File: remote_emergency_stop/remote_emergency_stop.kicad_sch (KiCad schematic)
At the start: 20 parts, among them J1 Conn_01x02, J2 Conn_01x02, Q1 BSS138, SW1 SW_DIP_x02, U1 MOUDLE-SEEEDUINO-XIAO-ESP32C3

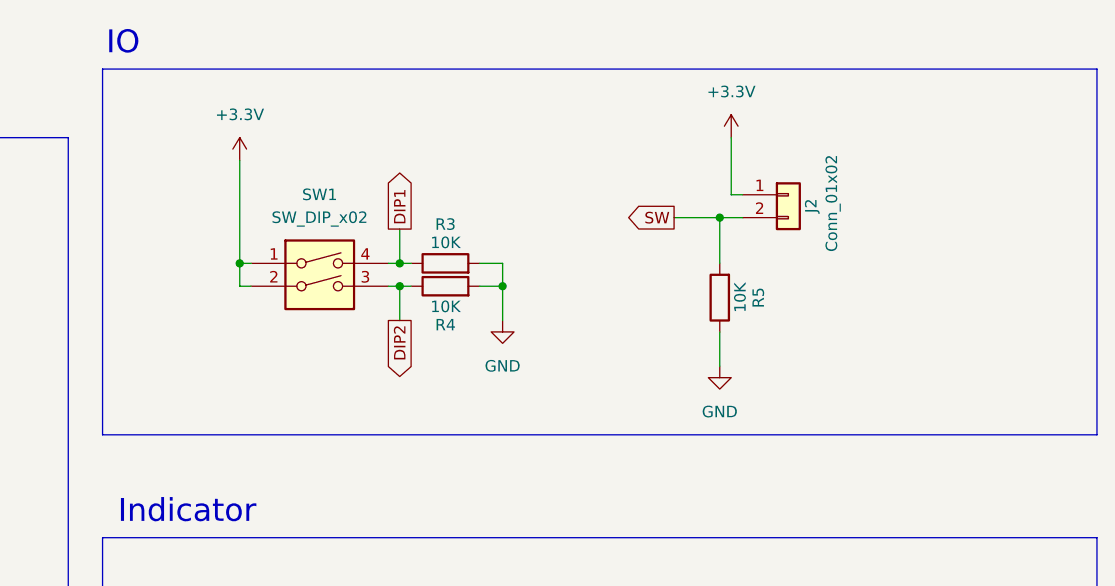
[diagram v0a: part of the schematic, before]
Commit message: 難しくてわかんないッピ
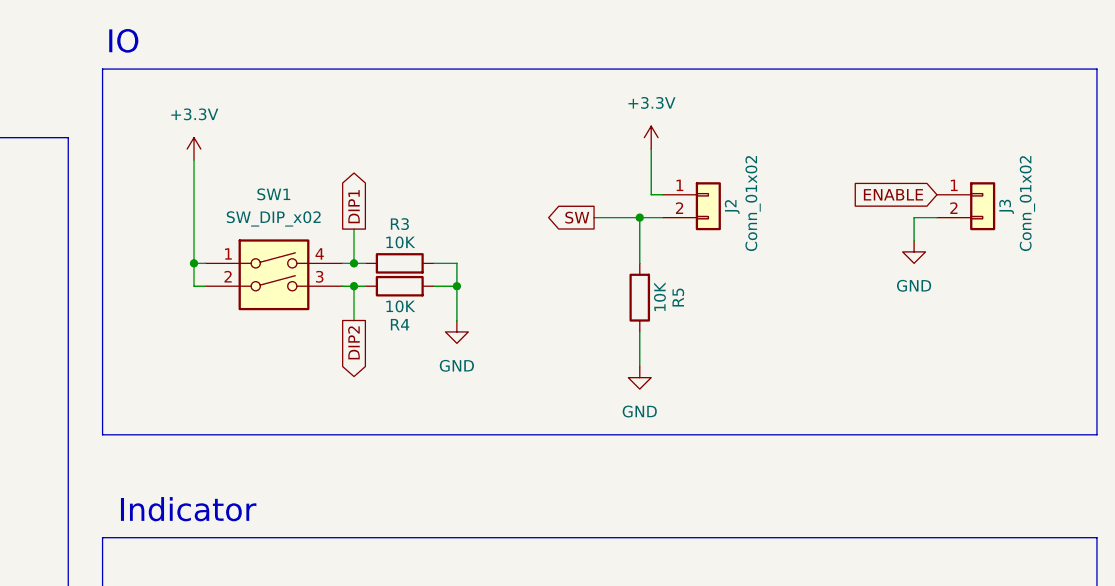
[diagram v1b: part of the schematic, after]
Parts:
- added J3: Conn_01x02, Connector_JST:JST_XH_S2B-XH-A_1x02_P2.50mm_Horizontal, symbol Connector_Generic:Conn_01x02
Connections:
- net ENABLE: now also J3.1 (Pin_1)
- net GND: now also J3.2 (Pin_2)
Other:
- moved on the sheet: J2, R3, R4, R5, SW1

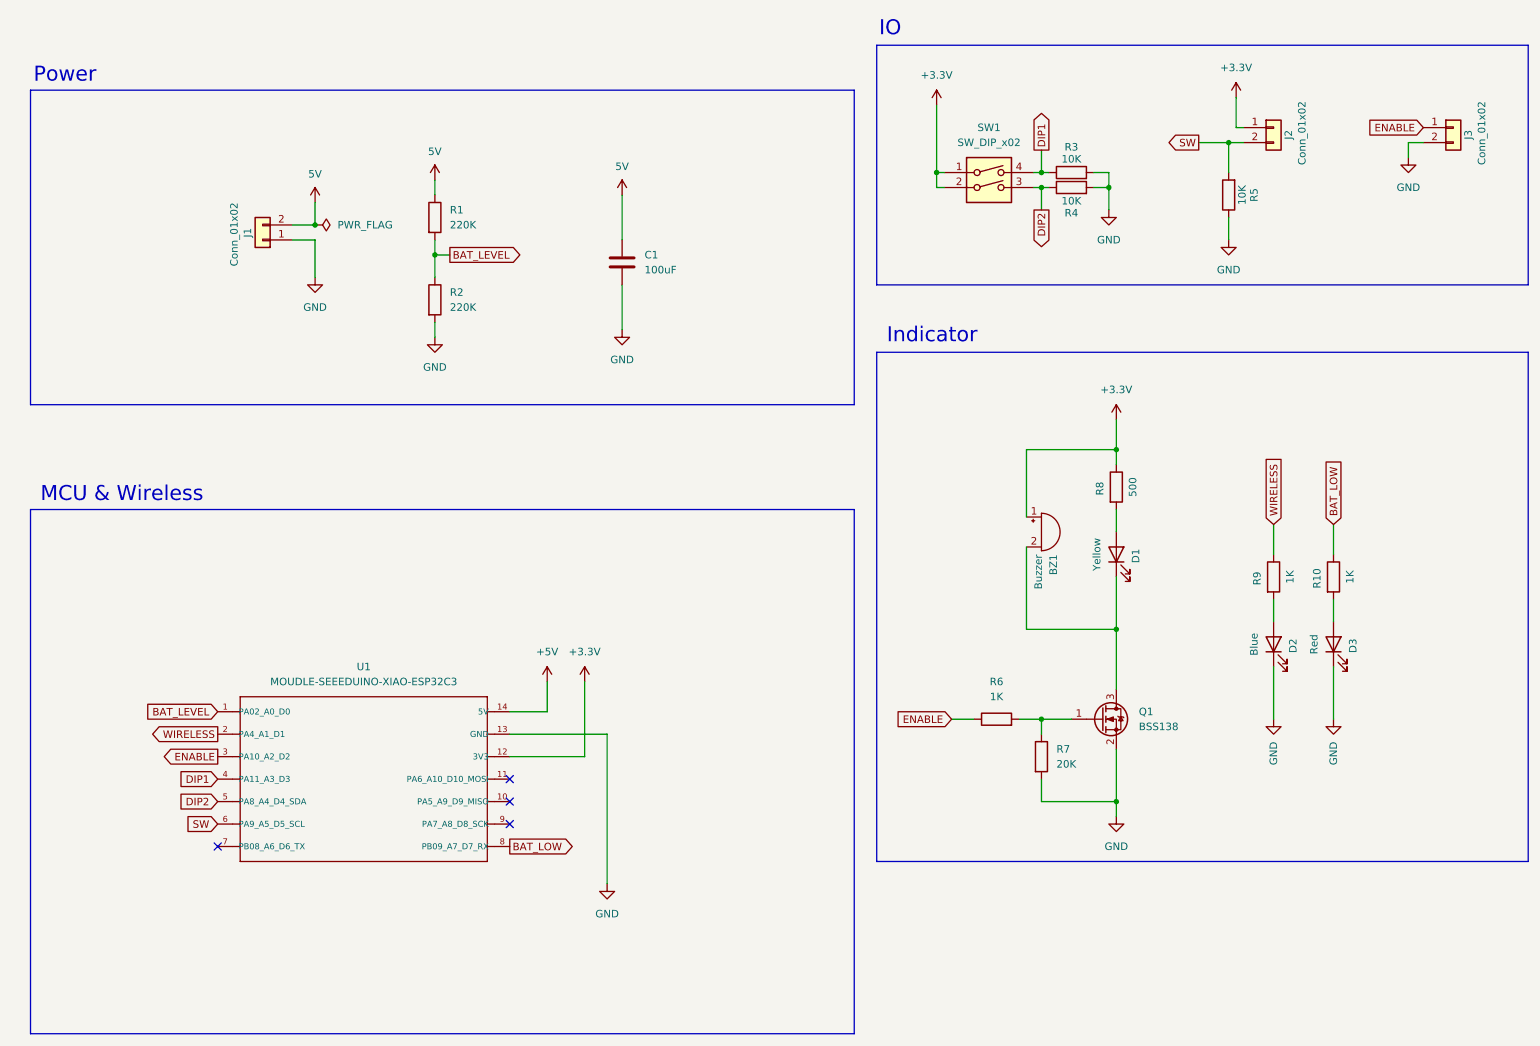
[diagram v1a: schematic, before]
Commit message: 尽きた
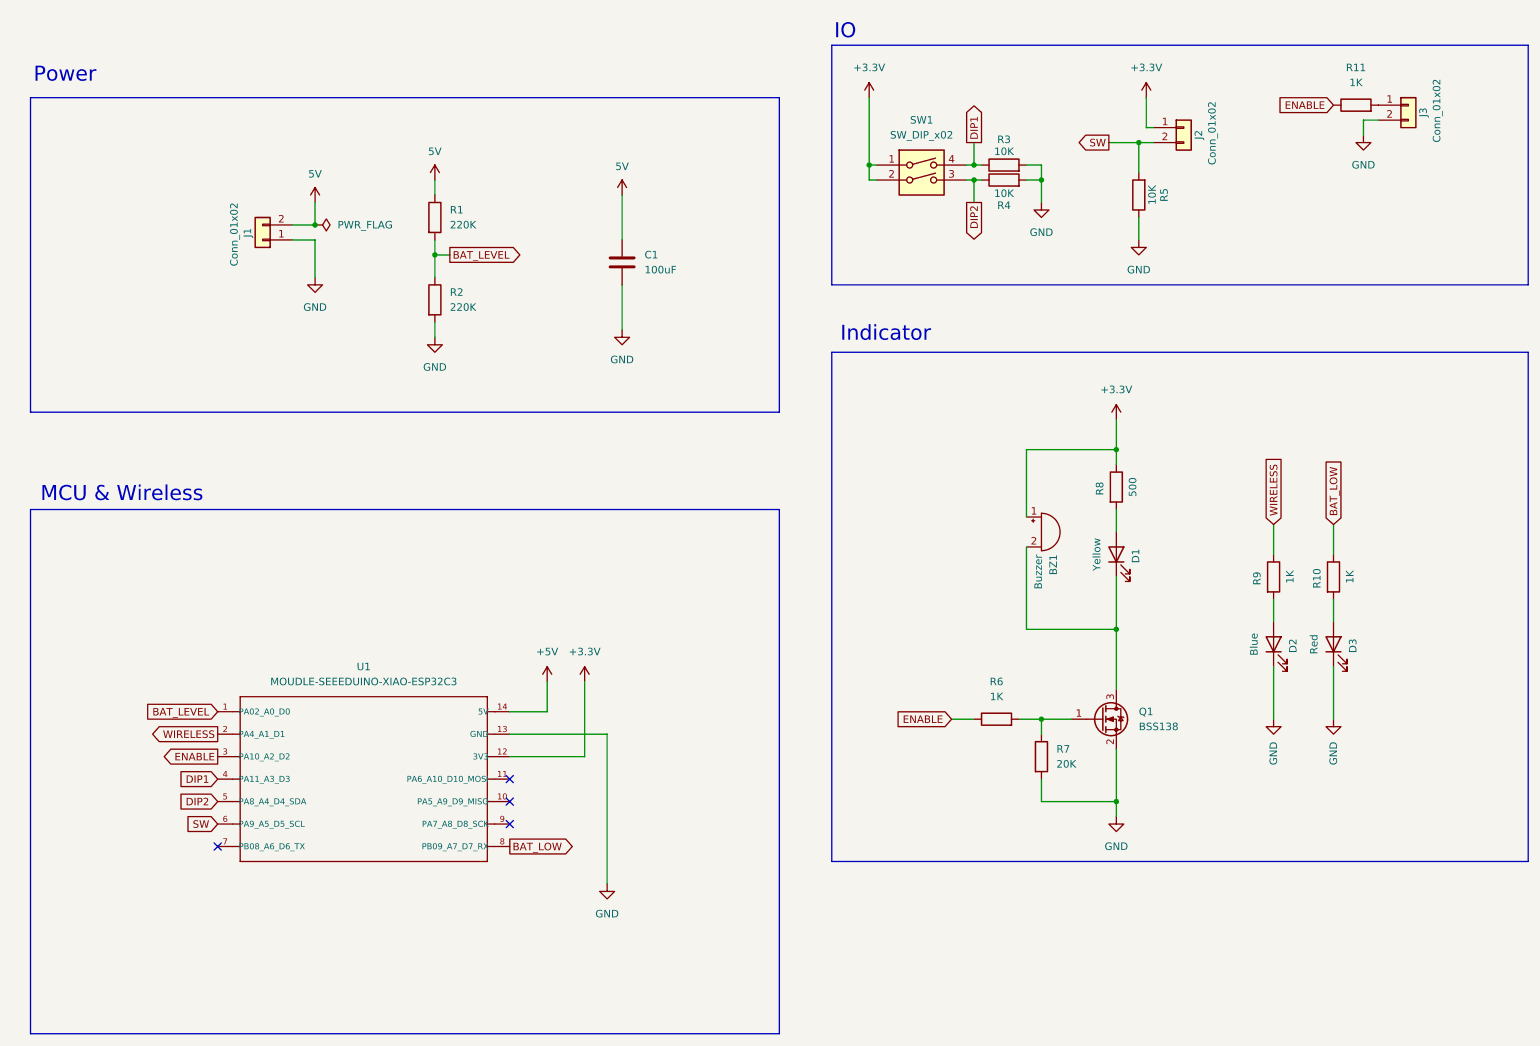
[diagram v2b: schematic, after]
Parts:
- added R11: 1K, symbol Device:R
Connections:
- net ENABLE: now also R11.1; no longer J3.1 (Pin_1)
- new net: J3.1 (Pin_1), R11.2
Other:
- moved on the sheet: J2, J3, R3, R4, R5, SW1
